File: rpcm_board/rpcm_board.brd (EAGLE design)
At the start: 65 x 56 mm, 37 parts, among them IC1 V7805-1000, Q1 IRLML6346TRPBF, U1 AL5812MP-13, U2 TB6621FNG

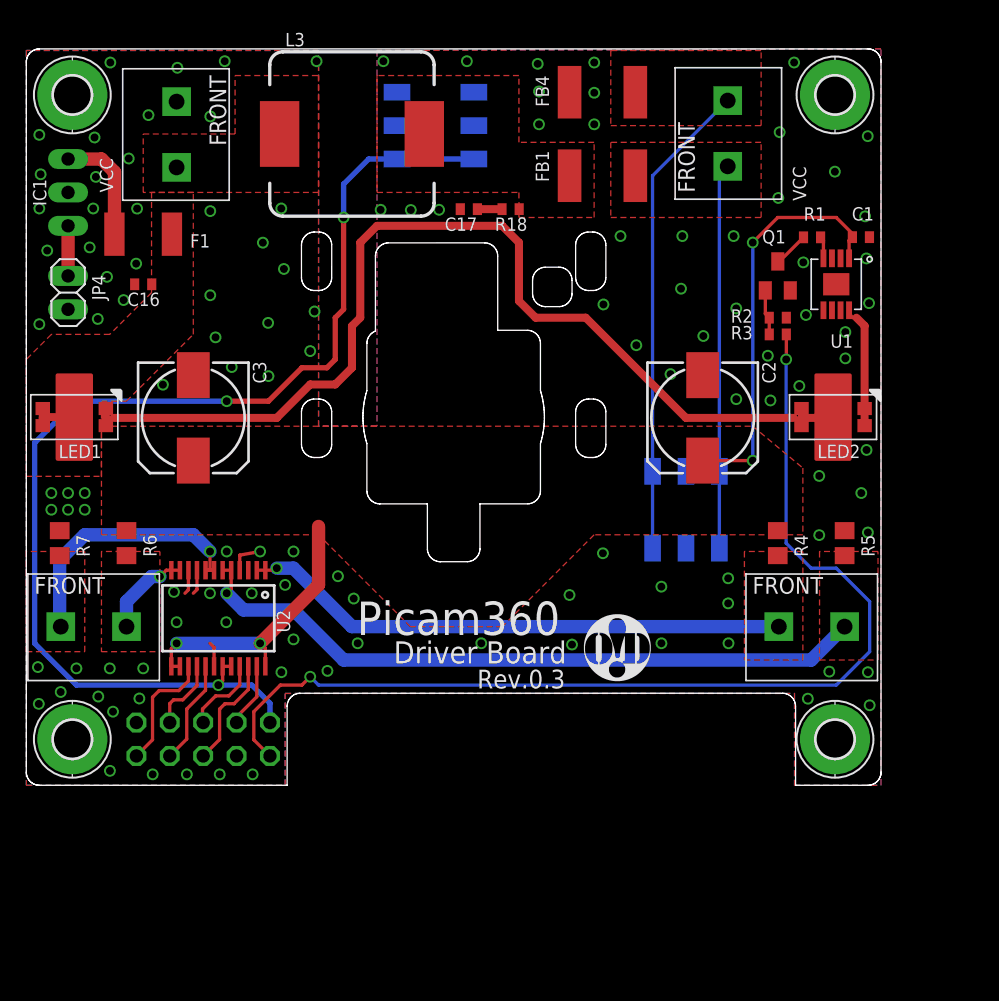
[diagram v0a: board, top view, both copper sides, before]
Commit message: refactoring
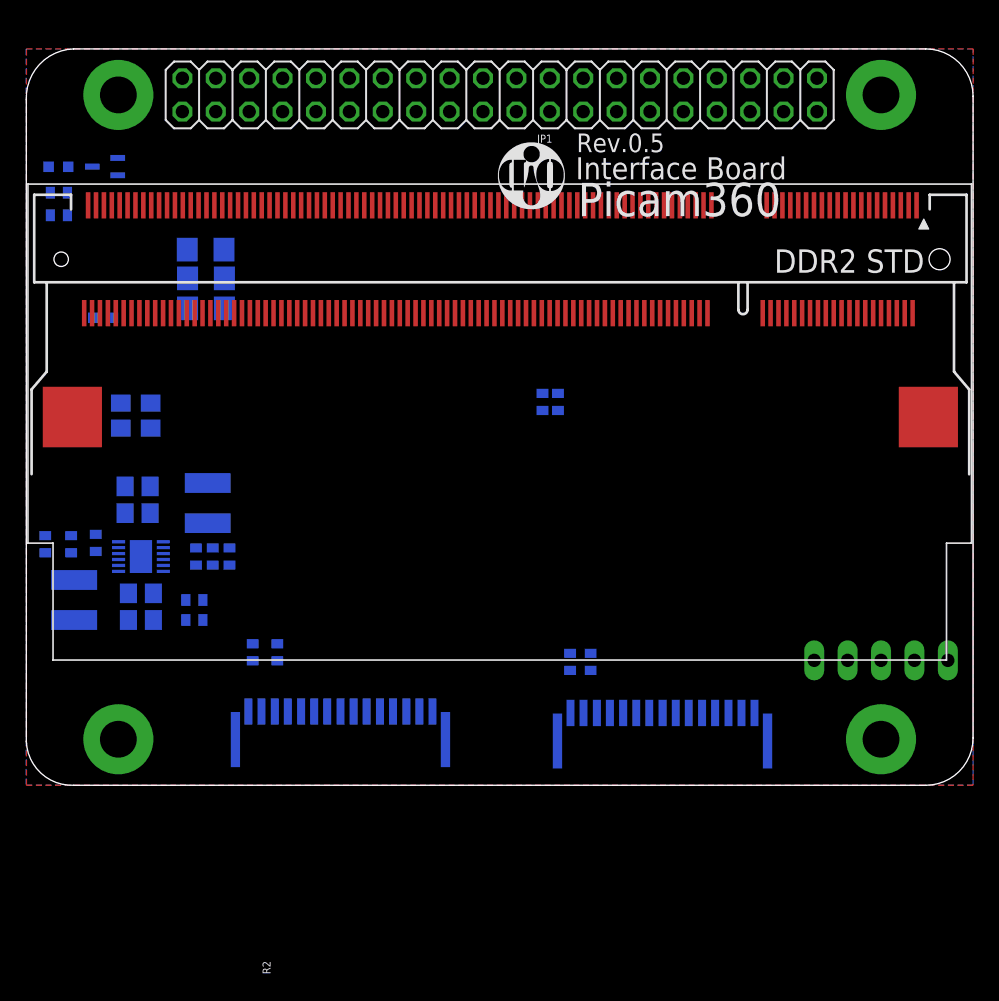
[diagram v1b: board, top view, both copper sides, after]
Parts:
- removed C16: 1u, resistor:C0402
- removed C17: 10n, resistor:C0402
- removed F1: MF-MSMF200-2, openblw:1812
- removed FB1, FB4: HR2220V801R-10, resistor:L5650M
- removed IC1: V7805-1000, openblw:DIP_3PIN
- removed JP3: M20-9980346, pinhead+:2X03_SMT
- removed JP4: (no value), pinhead:1X02
- removed L3: SRP1245A-100M, openblw:SRP1250A
- removed Q1: IRLML6346TRPBF, openblw:SOT23
- removed R18: 1K, resistor:R0402
- removed U$2, U$4, U$7, U$8: 282836-2, openblw:282836-2
- removed U$3: (no value), openblw:TENDA_P200
- added C12, C13, C14: 47u, resistor:C1206
- added C4, C5: 100p, resistor:C0402
- added C6, C7: 10u, resistor:C0805
- added L1, L2: SRN4018-4R7M(4.7u), openblw:BOURNS-SRN4018
- added PCB1: 1473005-4, openblw:RPI_COMPUTE
- added R11, R12: 100K, resistor:R0402
- added R13, R14, R16, R17: 1.8K, resistor:R0402
- added R15: 470R, resistor:R0402
- added R8, R9: 0R, resistor:R0805
- added U3: DMG1012T, openblw:SOT523
- added U5: PAM2306DYPAA, openblw:WDFN3X3-12L
- C2, C3: value UWT1E221MNL1GS(220u) -> 10u; device resistor:153CLV-0810 -> resistor:C0805
- JP1: value M20-9990446 -> M20-9980446; device pinhead:2X05 -> pinhead:2X20
- JP2: value M20-9980346 -> (none); device pinhead+:2X03_SMT -> pinhead:1X05
- LED1: value LTW-5630AZL50 -> RED; device openblw:LITEON-5630 -> led:CHIP-LED0603
- LED2: value LTW-5630AZL50 -> GREEN; device openblw:LITEON-5630 -> led:CHIP-LED0603
- R1: value 4.99K -> 100K
- R2: value 100K -> 450K
- R3: value 1K -> 200K
- R4, R5: value (none) -> 100K; device resistor:R0805 -> resistor:R0402
- R6: value (none) -> 470R; device resistor:R0805 -> resistor:R0402
- R7: value (none) -> 0R
- U1: value AL5812MP-13 -> SFW15R-1STE1LF; device openblw:MSOP-8EP -> openblw:RPI_CAMERA
- U2: value TB6621FNG -> SFW15R-1STE1LF; device openblw:SSOP24 -> openblw:RPI_CAMERA
- moved H3 78.6 mm to (65.0, 3.50), flipped to the bottom, turned to 180 degrees
- moved H4 73.3 mm to (7.00, 3.50), flipped to the bottom, turned to 180 degrees
- moved LED2 61.9 mm to (2.44, 47.0), flipped to the bottom, turned to 90 degrees
- moved R5 60.8 mm to (1.44, 18.3), flipped to the bottom, turned to 90 degrees
- moved C1 58.5 mm to (12.8, 12.6), flipped to the bottom
- moved R2 54.6 mm to (5.28, 18.4), flipped to the bottom, turned to 270 degrees
- moved R1 54.5 mm to (12.8, 14.1), flipped to the bottom
- moved JP1 53.9 mm to (36.0, 52.5), flipped to the top
- moved H1 49.1 mm to (7.00, 52.5), flipped to the bottom, turned to 180 degrees
- moved H2 49.1 mm to (65.0, 52.5), flipped to the bottom, turned to 180 degrees
- moved R3 47.4 mm to (12.9, 17.4), flipped to the bottom, turned to 90 degrees
- moved C2 43.6 mm to (8.46, 20.7), flipped to the bottom, turned to 0 degrees
- moved R4 41.7 mm to (15.4, 17.4), flipped to the bottom
- moved LOGO1 36.6 mm to (38.4, 46.4), turned to 180 degrees
- moved U1 32.6 mm to (48.4, 8.25), flipped to the bottom
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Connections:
- removed net +12V: C1.2, C16.1, C2.+, C3.+, F1.1, L3.2, LED1.A1, LED1.A2, LED1.A3, R4.1, R6.1, U$4.CON2, U1.1, U2.13, U2.14, U2.24
- removed net AGND: FB4.1, JP2.5, JP2.6, U$2.CON2
- removed net AIN1: JP1.6, U2.21
- removed net AIN2: JP1.5, U2.22
- removed net AOUT1: R4.2, U$8.CON1, U2.1, U2.2
- removed net AOUT2: R5.2, U$8.CON2, U2.5, U2.6
- removed net AVCC: FB1.1, JP2.1, JP2.2, U$2.CON1
- removed net BIN1: JP1.7, U2.17
- removed net BIN2: JP1.8, U2.16
- removed net BOUT1: R6.2, U$7.CON2, U2.11, U2.12
- removed net BOUT2: R7.2, U$7.CON1, U2.7, U2.8
- removed net LIGHT_PWM: JP1.1, R3.2
- removed net N$38: C17.1, R18.2
- removed net N$39: F1.2, IC1.IN
- removed net N$5: R1.2, U1.4
- removed net N$6: Q1.3, R1.1
- removed net PWMA: JP1.4, U2.23
- removed net PWMB: JP1.9, U2.15
- new net +1V8: C5.1, C7.1, JP2.1, L2.P$1, R3.1, R9.2
- new net BOTTOM_LIGHT_ENABLED: PCB1.59
- new net CAM0_C_N: PCB1.144, U1.8
- new net CAM0_C_P: PCB1.142, U1.9
- new net CAM0_D0_N: PCB1.138, U1.2
- new net CAM0_D0_P: PCB1.136, U1.3
- new net CAM0_D1_N: PCB1.150, U1.5
- new net CAM0_D1_P: PCB1.148, U1.6
- new net CAM0_IO0: PCB1.36, U1.11
- new net CAM0_IO1: PCB1.34, U1.12
- new net CAM0_SCL: PCB1.30, R13.1, U1.13
- new net CAM0_SDA: PCB1.28, R14.1, U1.14
- new net CAM1_C_N: PCB1.149, U2.8
- new net CAM1_C_P: PCB1.147, U2.9
- new net CAM1_D0_N: PCB1.161, U2.2
- new net CAM1_D0_P: PCB1.159, U2.3
- new net CAM1_D1_N: PCB1.155, U2.5
- new net CAM1_D1_P: PCB1.153, U2.6
- new net CAM1_IO0: PCB1.11, U2.11
- new net CAM1_IO1: PCB1.9, U2.12
- new net CAM1_SCL: PCB1.5, R17.1, U2.13
- new net CAM1_SDA: PCB1.3, R16.1, U2.14
- new net CM_1V8: C12.1, PCB1.183, PCB1.184, PCB1.185, PCB1.186, R9.1
- new net CM_3V3: C13.1, PCB1.189, PCB1.190, PCB1.191, PCB1.192, PCB1.193, PCB1.194, R8.1
- new net CM_VBAT: C14.1, PCB1.197, PCB1.198, PCB1.199, PCB1.200, R7.1
- new net EMMC_DISABLE_N: PCB1.2
- new net EXT0/UART1_TX: JP1.6, PCB1.70
- new net EXT1/UART1_RX: JP1.4, PCB1.72
- new net GPIO47_1V8: PCB1.90, U3.1
- new net LAN_RUN: PCB1.21
- new net N$10: C5.2, R3.2, R4.1, U5.10
- new net N$11: PCB1.154
- new net N$12: PCB1.156
- new net N$13: PCB1.158
- new net N$14: PCB1.160
- new net N$15: PCB1.162
- new net N$16: PCB1.10
- new net N$17: PCB1.12
- new net N$18: PCB1.14
- new net N$19: PCB1.16
- new net N$2: L1.P$2, U5.8
- new net N$20: PCB1.18
- new net N$21: PCB1.20
- new net N$22: PCB1.22
- new net N$23: PCB1.24
- new net N$24: PCB1.124
- new net N$25: PCB1.126
- new net N$26: PCB1.128
- new net N$27: PCB1.130
- new net N$28: PCB1.132
- new net N$29: PCB1.4
- new net N$30: PCB1.6
- new net N$31: PCB1.82, R12.1
- new net N$32: LED2.A, R15.2
- new net N$33: LED2.C, U3.3
- new net N$34: PCB1.84, R11.1
- new net N$35: PCB1.8
- new net N$4: U5.11
- new net N$8: C4.2, R2.2, R5.1, U5.4
- new net TOP_LIGHT_ENABLED: PCB1.57
- new net UART0_RX: JP1.5, PCB1.53
- new net UART0_TX: JP1.3, PCB1.51
- new net USB_D_N: JP2.4, PCB1.167
- new net USB_D_P: JP2.3, PCB1.165
- net +3V3: now also C4.1, C6.1, L1.P$1, PCB1.39, PCB1.40, PCB1.41, PCB1.42, R13.2, R14.2, R15.1, R16.2, R17.2, R2.1, R6.1, R7.2, R8.2, U1.15, U2.15; no longer JP1.2, JP3.5, JP3.6, U2.19, U2.20
- net +5V: now also C2.1, C3.1, JP1.1, JP1.2, JP2.2, R1.1, U5.1, U5.6, U5.7; no longer IC1.OUT, JP4.1
- net GND: now also C1.2, C12.2, C13.2, C14.2, C2.2, C3.2, C6.2, C7.2, JP1.13, JP1.14, JP1.7, JP1.8, JP2.5, LED1.C, PCB1.1, PCB1.103, PCB1.104, PCB1.109, PCB1.110, PCB1.115, PCB1.121, PCB1.122, PCB1.127, PCB1.13, PCB1.133, PCB1.134, PCB1.139, PCB1.140, PCB1.145, PCB1.146, PCB1.151, PCB1.152, PCB1.157, PCB1.163, PCB1.164, PCB1.168, PCB1.169, PCB1.170, PCB1.181, PCB1.182, PCB1.187, PCB1.188, PCB1.19, PCB1.195, PCB1.196, PCB1.25, PCB1.26, PCB1.31, PCB1.32, PCB1.37, PCB1.38, PCB1.43, PCB1.44, PCB1.49, PCB1.50, PCB1.55, PCB1.56, PCB1.61, PCB1.62, PCB1.67, PCB1.68, PCB1.7, PCB1.73, PCB1.74, PCB1.79, PCB1.80, PCB1.85, PCB1.86, PCB1.91, PCB1.92, PCB1.97, PCB1.98, R11.2, R12.2, R4.2, R5.2, U1.1, U1.10, U1.4, U1.7, U2.1, U2.7, U3.2, U5.3, U5.9, U5.PAD; no longer C1.1, C16.2, C17.2, C2.-, C3.-, FB4.2, IC1.GND, JP1.10, JP1.3, JP3.1, JP4.2, Q1.2, R2.1, R5.1, R7.1, U$4.CON1, U1.5, U1.HSINK, U2.18, U2.3, U2.9
- net N$1: now also C1.1, R1.2, U5.12; no longer LED1.C1, LED1.C2, LED2.A1, LED2.A2, LED2.A3
- net N$3: now also U5.5; no longer FB1.2, L3.1, R18.1
- net N$7: now also L2.P$2, U5.2; no longer Q1.1, R2.2, R3.1
- net N$9: now also LED1.A, R6.2; no longer LED2.C1, LED2.C2, U1.8
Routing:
- net +3V3: track 88.5 -> 0.00 mm, vias 3 -> 0
- net LIGHT_PWM: track 81.0 -> 0.00 mm, vias 2 -> 0
- net N$1: track 78.9 -> 0.00 mm
- net +12V: track 58.1 -> 0.00 mm, vias 4 -> 0
- net AOUT2: track 52.7 -> 0.00 mm, vias 1 -> 0
- net AOUT1: track 41.6 -> 0.00 mm, vias 1 -> 0
- net AGND: track 36.4 -> 0.00 mm
- net AVCC: track 29.3 -> 0.00 mm
- net BOUT2: track 20.3 -> 0.00 mm, vias 1 -> 0
- net N$9: track 9.42 -> 0.00 mm
- net PWMB: track 9.33 -> 0.00 mm
- net N$39: track 8.67 -> 0.00 mm
- net AIN2: track 8.64 -> 0.00 mm
- net GND: track 8.33 -> 0.00 mm, vias 122 -> 0
- net BIN1: track 7.94 -> 0.00 mm
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- added copper zone on layer 15, net GND
- added copper zone on layer 2, net GND
- removed copper zone on layer 1, net +12V
- removed copper zone on layer 1, net AGND
- removed copper zone on layer 1, net AOUT1
- removed copper zone on layer 1, net AOUT2
- removed copper zone on layer 1, net AVCC
- removed copper zone on layer 1, net BOUT1
- removed copper zone on layer 1, net BOUT2
- removed copper zone on layer 1, net N$3
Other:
- board size 65 x 56 mm -> 72 x 56 mm
- board text added: "*"
- board text added: "AVCC"
- board text added: "CAM0"
- board text added: "CAM1"
- board text added: "Interface Board"
- board text added: "Rev.0.5"
- board text removed: "Driver Board"
- board text removed: "Rev.0.3"
